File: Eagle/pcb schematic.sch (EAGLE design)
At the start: 17 parts

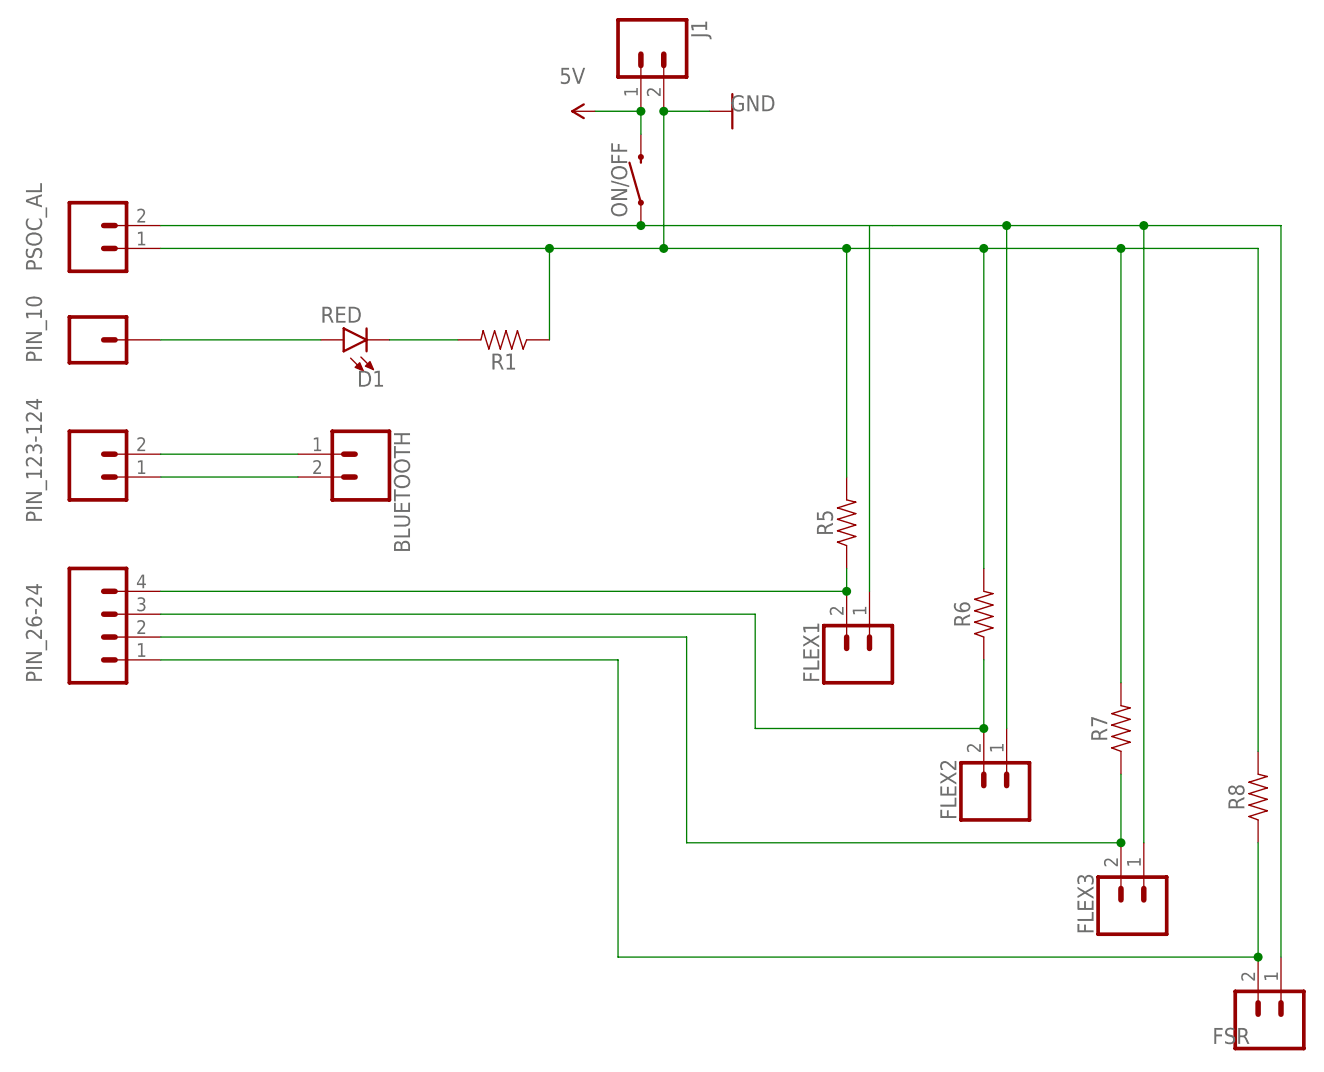
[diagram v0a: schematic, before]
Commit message: PCB finita
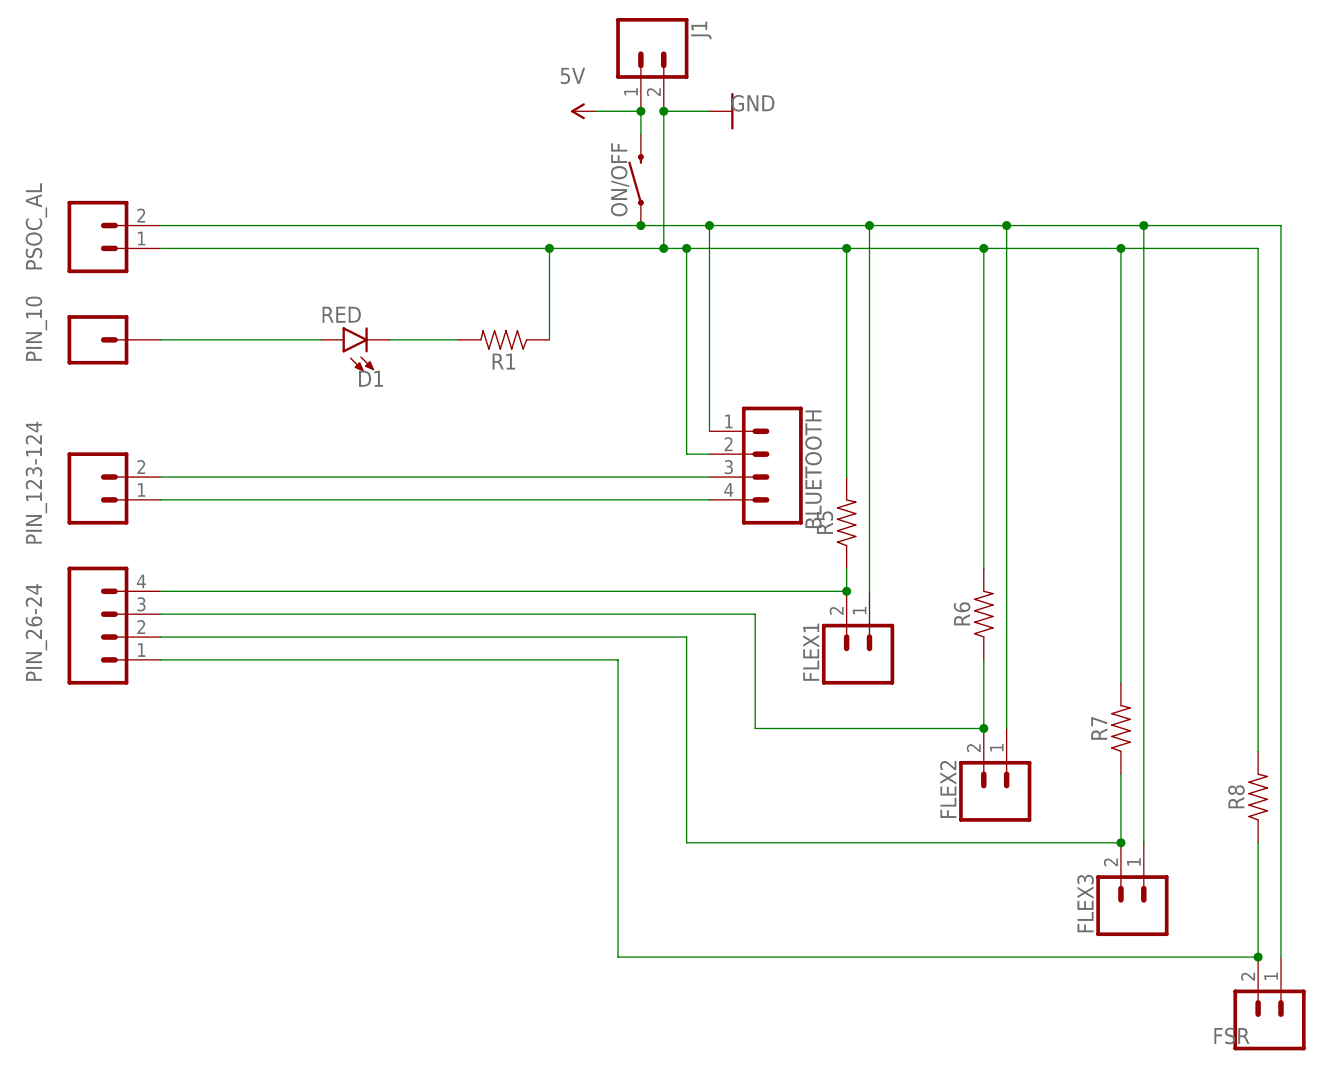
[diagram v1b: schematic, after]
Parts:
- BLUETOOTH: device SparkFun-Connectors:CONN_02 -> SparkFun-Connectors:CONN_04
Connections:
- net GND: now also BLUETOOTH.2
- net N$4: now also BLUETOOTH.4, PIN_123-124.1; no longer BLUETOOTH.1, PIN_123-124.2
- net N$6: now also BLUETOOTH.3, PIN_123-124.2; no longer BLUETOOTH.2, PIN_123-124.1
- net N$9: now also BLUETOOTH.1
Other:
- moved on the sheet: PIN_123-124
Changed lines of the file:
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@@
 <part name="R1" library="SparkFun-Resistors" deviceset="RESISTOR" device="AXIAL-0.3" value=" "/>
 <part name="PIN_123-124" library="SparkFun-Connectors" deviceset="CONN_02" device=""/>
-<part name="BLUETOOTH" library="SparkFun-Connectors" deviceset="CONN_02" device=""/>
 <part name="J1" library="SparkFun-Connectors" deviceset="CONN_02" device=""/>
+<part name="BLUETOOTH" library="SparkFun-Connectors" deviceset="CONN_04" device=""/>
 </parts>
 <sheets>
@@
 <attribute name="NAME" x="-10.16" y="61.976" size="1.778" layer="95" font="vector" rot="R180" align="bottom-center"/>
 </instance>
-<instance part="PIN_123-124" gate="G$1" x="-55.88" y="48.26" smashed="yes">
-<attribute name="VALUE" x="-58.42" y="43.434" size="1.778" layer="96" font="vector"/>
-<attribute name="NAME" x="-61.468" y="43.18" size="1.778" layer="95" font="vector" rot="R90"/>
-</instance>
-<instance part="BLUETOOTH" gate="G$1" x="-25.4" y="50.8" smashed="yes" rot="R180">
-<attribute name="VALUE" x="-22.86" y="55.626" size="1.778" layer="96" font="vector" rot="R180"/>
-<attribute name="NAME" x="-22.352" y="53.34" size="1.778" layer="95" font="vector" rot="R270"/>
+<instance part="PIN_123-124" gate="G$1" x="-55.88" y="45.72" smashed="yes">
+<attribute name="VALUE" x="-58.42" y="40.894" size="1.778" layer="96" font="vector"/>
+<attribute name="NAME" x="-61.468" y="40.64" size="1.778" layer="95" font="vector" rot="R90"/>
 </instance>
 <instance part="J1" gate="G$1" x="5.08" y="96.52" smashed="yes" rot="R270">
 <attribute name="VALUE" x="0.254" y="99.06" size="1.778" layer="96" font="vector" rot="R270"/>
 <attribute name="NAME" x="10.668" y="99.06" size="1.778" layer="95" font="vector" rot="R270"/>
+</instance>
+<instance part="BLUETOOTH" gate="G$1" x="17.78" y="50.8" smashed="yes" rot="R180">
+<attribute name="VALUE" x="22.86" y="58.166" size="1.778" layer="96" font="vector" rot="R180"/>
+<attribute name="NAME" x="23.368" y="55.88" size="1.778" layer="95" font="vector" rot="R270"/>
 </instance>
 </instances>
@@
 <wire x1="-48.26" y1="76.2" x2="5.08" y2="76.2" width="0.1524" layer="91"/>
 <pinref part="FLEX2" gate="G$1" pin="1"/>
-<wire x1="30.48" y1="76.2" x2="33.02" y2="76.2" width="0.1524" layer="91"/>
-<wire x1="33.02" y1="76.2" x2="45.72" y2="76.2" width="0.1524" layer="91"/>
 <wire x1="45.72" y1="20.32" x2="45.72" y2="76.2" width="0.1524" layer="91"/>
 <wire x1="45.72" y1="76.2" x2="60.96" y2="76.2" width="0.1524" layer="91"/>
@@
 <wire x1="60.96" y1="7.62" x2="60.96" y2="76.2" width="0.1524" layer="91"/>
 <junction x="60.96" y="76.2"/>
+<wire x1="5.08" y1="76.2" x2="12.7" y2="76.2" width="0.1524" layer="91"/>
+<junction x="5.08" y="76.2"/>
+<pinref part="BLUETOOTH" gate="G$1" pin="1"/>
+<wire x1="12.7" y1="76.2" x2="30.48" y2="76.2" width="0.1524" layer="91"/>
+<wire x1="30.48" y1="76.2" x2="45.72" y2="76.2" width="0.1524" layer="91"/>
+<wire x1="12.7" y1="53.34" x2="12.7" y2="76.2" width="0.1524" layer="91"/>
+<junction x="12.7" y="76.2"/>
 <pinref part="FLEX1" gate="G$1" pin="1"/>
 <wire x1="30.48" y1="35.56" x2="30.48" y2="76.2" width="0.1524" layer="91"/>
-<wire x1="5.08" y1="76.2" x2="30.48" y2="76.2" width="0.1524" layer="91"/>
-<junction x="5.08" y="76.2"/>
+<junction x="30.48" y="76.2"/>
 </segment>
 </net>
@@
 <pinref part="R1" gate="G$1" pin="2"/>
 <wire x1="-22.86" y1="63.5" x2="-15.24" y2="63.5" width="0.1524" layer="91"/>
-</segment>
-</net>
-<net name="N$4" class="0">
-<segment>
-<pinref part="PIN_123-124" gate="G$1" pin="2"/>
-<pinref part="BLUETOOTH" gate="G$1" pin="1"/>
-<wire x1="-48.26" y1="50.8" x2="-33.02" y2="50.8" width="0.1524" layer="91"/>
-</segment>
-</net>
-<net name="N$6" class="0">
-<segment>
-<pinref part="PIN_123-124" gate="G$1" pin="1"/>
-<pinref part="BLUETOOTH" gate="G$1" pin="2"/>
-<wire x1="-48.26" y1="48.26" x2="-33.02" y2="48.26" width="0.1524" layer="91"/>
 </segment>
 </net>
@@
 <pinref part="R5" gate="G$1" pin="2"/>
 <wire x1="27.94" y1="73.66" x2="27.94" y2="48.26" width="0.1524" layer="91"/>
-<wire x1="7.62" y1="73.66" x2="27.94" y2="73.66" width="0.1524" layer="91"/>
+<wire x1="7.62" y1="73.66" x2="10.16" y2="73.66" width="0.1524" layer="91"/>
 <junction x="27.94" y="73.66"/>
 <pinref part="R1" gate="G$1" pin="1"/>
+<wire x1="10.16" y1="73.66" x2="27.94" y2="73.66" width="0.1524" layer="91"/>
 <wire x1="-5.08" y1="63.5" x2="-5.08" y2="73.66" width="0.1524" layer="91"/>
 <wire x1="-48.26" y1="73.66" x2="-5.08" y2="73.66" width="0.1524" layer="91"/>
@@
 <junction x="7.62" y="73.66"/>
 <junction x="-5.08" y="73.66"/>
-</segment>
-</net>
+<pinref part="BLUETOOTH" gate="G$1" pin="2"/>
+<wire x1="12.7" y1="50.8" x2="10.16" y2="50.8" width="0.1524" layer="91"/>
+<wire x1="10.16" y1="50.8" x2="10.16" y2="73.66" width="0.1524" layer="91"/>
+<junction x="10.16" y="73.66"/>
+</segment>
+</net>
+<net name="N$4" class="0">
+<segment>
+<pinref part="PIN_123-124" gate="G$1" pin="1"/>
+<pinref part="BLUETOOTH" gate="G$1" pin="4"/>
+<wire x1="-48.26" y1="45.72" x2="12.7" y2="45.72" width="0.1524" layer="91"/>
+</segment>
+</net>
+<net name="N$6" class="0">
+<segment>
+<pinref part="PIN_123-124" gate="G$1" pin="2"/>
+<pinref part="BLUETOOTH" gate="G$1" pin="3"/>
+<wire x1="-48.26" y1="48.26" x2="12.7" y2="48.26" width="0.1524" layer="91"/>
+</segment>
+</net>
